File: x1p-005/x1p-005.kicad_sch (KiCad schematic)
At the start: 72 parts, among them Q1 LMBT3904LT1G, SW1 6.0*6.0*6.0, SW2 6.0*6.0*6.0, U1 AD24C02, U2 SN74LVC1T45DBVR, U4 SN74LVC1G3157DBVR_C3040658, U5 SN74LVC1G3157DBVR_C3040658

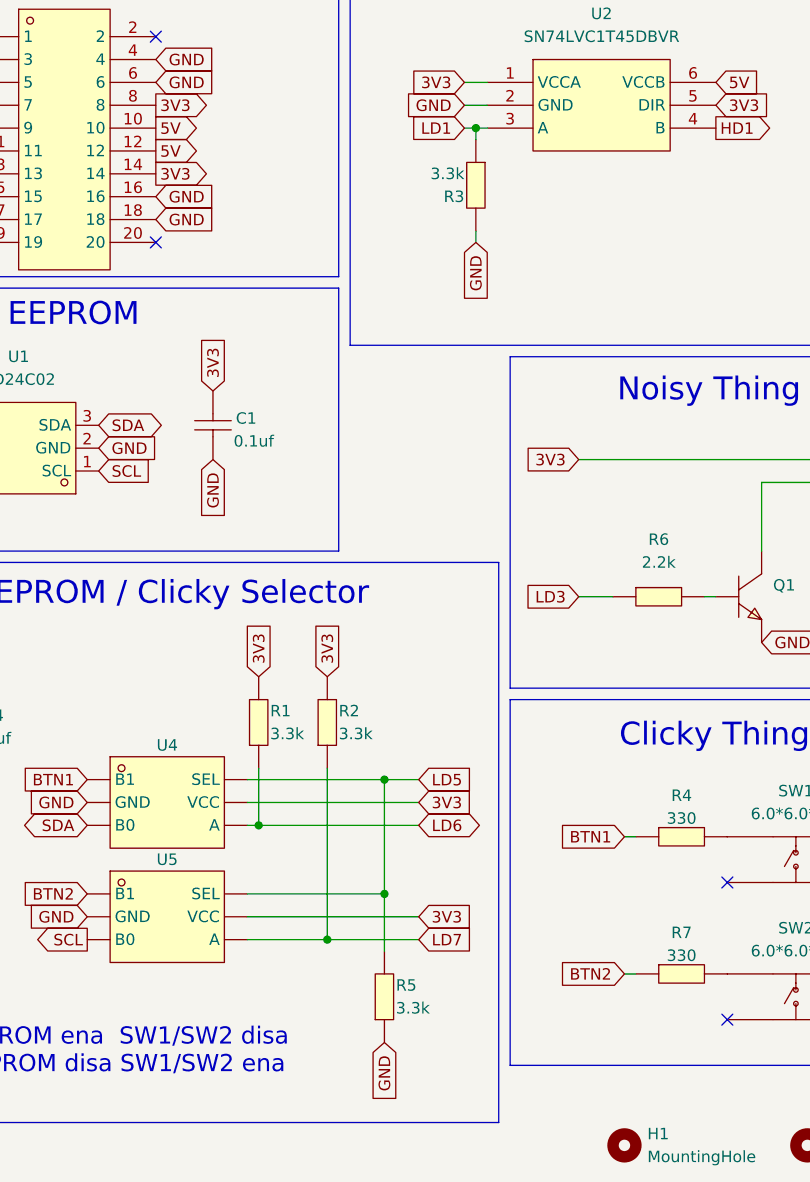
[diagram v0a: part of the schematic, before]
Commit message: x1p-005: resistors to 2.2k; remove a weird dangling trace; label beepies and clickies with their pin number
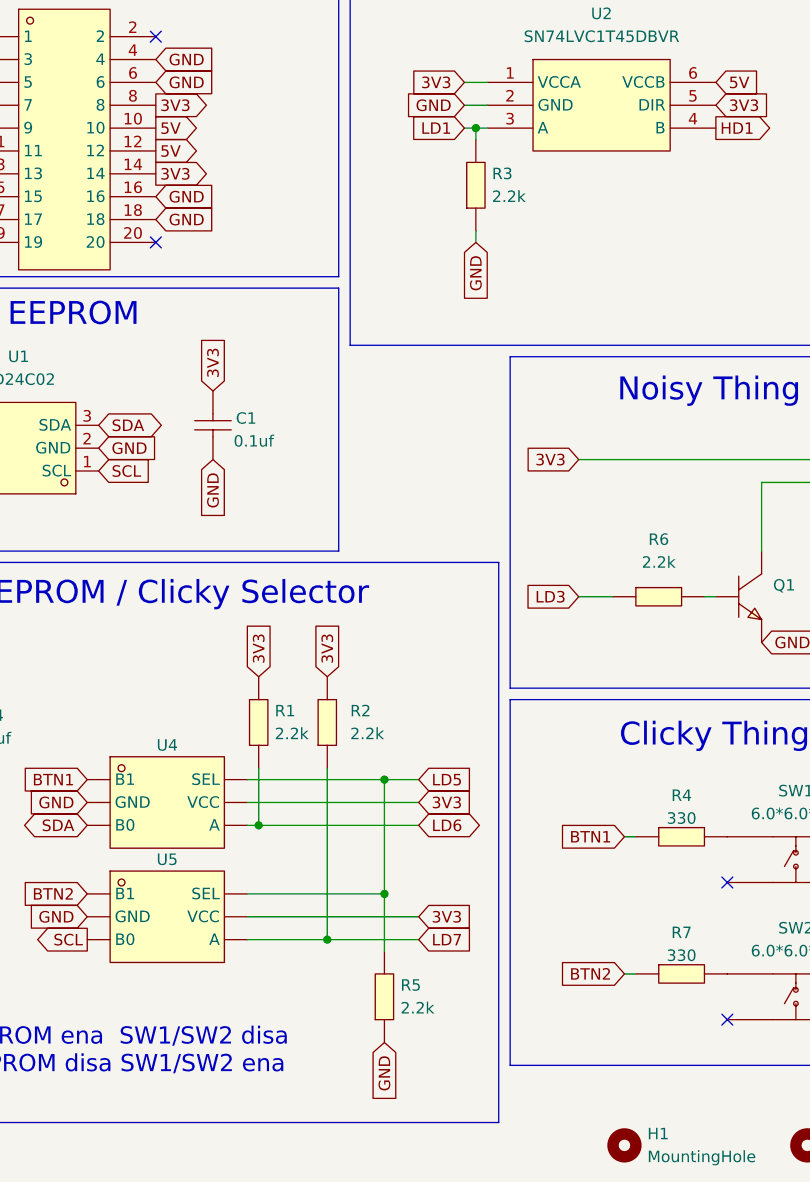
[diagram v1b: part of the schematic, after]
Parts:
- removed R1, R2, R5: 3.3k, x1p-005:R0402, symbol lcsc:0402WGF3301TCE
- removed R3: 3.3k, x1p-004:R0402, symbol lcsc:0402WGF3301TCE
- added R1, R2, R3, R5: 2.2k, x1p-005:R0402, symbol x1p-005:0402WGF2201TCE
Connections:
- net 3V3: now also R1.2, R2.2
- net GND: now also R3.1, R5.1
- net LD1: now also R3.2
- net LD5: now also R5.2
- net LD6: now also R1.1
- net LD7: now also R2.1

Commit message: x1p-005: fix up board layout to align with x1p-004
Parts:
- C1, C13, C14: footprint x1p-005:C0402 -> Capacitor_SMD:C_0402_1005Metric
- C10, C11, C12, C15, C16, C17, C18, C19, C2, C20, C21, C22, C23, C24, C25, C26, C27, C28, C29, C3, C4, C5, C6, C7, C8, C9: footprint x1p-004:C0402 -> Capacitor_SMD:C_0402_1005Metric
- R1, R2, R3, R4, R5, R6, R7: footprint x1p-005:R0402 -> Resistor_SMD:R_0402_1005Metric
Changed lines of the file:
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@@
 			)
 		)
-		(property "Footprint" "x1p-004:C0402"
+		(property "Footprint" "Capacitor_SMD:C_0402_1005Metric"
 			(at 204.47 137.16 0)
 			(effects
@@
 			)
 		)
-		(property "Footprint" "x1p-005:C0402"
+		(property "Footprint" "Capacitor_SMD:C_0402_1005Metric"
 			(at 19.05 101.6 0)
 			(effects
@@
 			)
 		)
-		(property "Footprint" "x1p-004:C0402"
+		(property "Footprint" "Capacitor_SMD:C_0402_1005Metric"
 			(at 247.65 137.16 0)
 			(effects
@@
 			)
 		)
-		(property "Footprint" "x1p-004:C0402"
+		(property "Footprint" "Capacitor_SMD:C_0402_1005Metric"
 			(at 166.37 137.16 0)
 			(effects
@@
 			)
 		)
-		(property "Footprint" "x1p-004:C0402"
+		(property "Footprint" "Capacitor_SMD:C_0402_1005Metric"
 			(at 166.37 149.86 0)
 			(effects
@@
 			)
 		)
-		(property "Footprint" "x1p-005:R0402"
+		(property "Footprint" "Resistor_SMD:R_0402_1005Metric"
 			(at 82.55 132.08 0)
 			(effects
@@
 			)
 		)
-		(property "Footprint" "x1p-004:C0402"
+		(property "Footprint" "Capacitor_SMD:C_0402_1005Metric"
 			(at 220.98 137.16 0)
 			(effects
@@
 			)
 		)
-		(property "Footprint" "x1p-004:C0402"
+		(property "Footprint" "Capacitor_SMD:C_0402_1005Metric"
 			(at 121.92 26.67 0)
 			(effects
@@
 			)
 		)
-		(property "Footprint" "x1p-004:C0402"
+		(property "Footprint" "Capacitor_SMD:C_0402_1005Metric"
 			(at 247.65 149.86 0)
 			(effects
@@
 			)
 		)
-		(property "Footprint" "x1p-005:R0402"
+		(property "Footprint" "Resistor_SMD:R_0402_1005Metric"
 			(at 92.71 41.91 0)
 			(effects
@@
 			)
 		)
-		(property "Footprint" "x1p-004:C0402"
+		(property "Footprint" "Capacitor_SMD:C_0402_1005Metric"
 			(at 189.23 137.16 0)
 			(effects
@@
 			)
 		)
-		(property "Footprint" "x1p-004:C0402"
+		(property "Footprint" "Capacitor_SMD:C_0402_1005Metric"
 			(at 256.54 149.86 0)
 			(effects
@@
 			)
 		)
-		(property "Footprint" "x1p-005:R0402"
+		(property "Footprint" "Resistor_SMD:R_0402_1005Metric"
 			(at 76.2 101.6 0)
 			(effects
@@
 			)
 		)
-		(property "Footprint" "x1p-004:C0402"
+		(property "Footprint" "Capacitor_SMD:C_0402_1005Metric"
 			(at 181.61 137.16 0)
 			(effects
@@
 			)
 		)
-		(property "Footprint" "x1p-005:R0402"
+		(property "Footprint" "Resistor_SMD:R_0402_1005Metric"
 			(at 107.95 137.16 0)
 			(effects
@@
 			)
 		)
-		(property "Footprint" "x1p-004:C0402"
+		(property "Footprint" "Capacitor_SMD:C_0402_1005Metric"
 			(at 220.98 149.86 0)
 			(effects
@@
 			)
 		)
-		(property "Footprint" "x1p-005:C0402"
+		(property "Footprint" "Capacitor_SMD:C_0402_1005Metric"
 			(at 10.16 101.6 0)
 			(effects
@@
 			)
 		)
-		(property "Footprint" "x1p-004:C0402"
+		(property "Footprint" "Capacitor_SMD:C_0402_1005Metric"
 			(at 158.75 149.86 0)
 			(effects
@@
 			)
 		)
-		(property "Footprint" "x1p-004:C0402"
+		(property "Footprint" "Capacitor_SMD:C_0402_1005Metric"
 			(at 189.23 149.86 0)
 			(effects
@@
 			)
 		)
-		(property "Footprint" "x1p-005:C0402"
+		(property "Footprint" "Capacitor_SMD:C_0402_1005Metric"
 			(at 48.26 68.58 0)
 			(effects
@@
 			)
 		)
-		(property "Footprint" "x1p-004:C0402"
+		(property "Footprint" "Capacitor_SMD:C_0402_1005Metric"
 			(at 204.47 149.86 0)
 			(effects
@@
 			)
 		)
-		(property "Footprint" "x1p-004:C0402"
+		(property "Footprint" "Capacitor_SMD:C_0402_1005Metric"
 			(at 212.09 137.16 0)
 			(effects
@@
 			)
 		)
-		(property "Footprint" "x1p-004:C0402"
+		(property "Footprint" "Capacitor_SMD:C_0402_1005Metric"
 			(at 212.09 149.86 0)
 			(effects
@@
 			)
 		)
-		(property "Footprint" "x1p-004:C0402"
+		(property "Footprint" "Capacitor_SMD:C_0402_1005Metric"
 			(at 238.76 149.86 0)
 			(effects
@@
 			)
 		)
-		(property "Footprint" "x1p-005:R0402"
+		(property "Footprint" "Resistor_SMD:R_0402_1005Metric"
 			(at 105.41 95.25 0)
 			(effects
@@
 			)
 		)
-		(property "Footprint" "x1p-004:C0402"
+		(property "Footprint" "Capacitor_SMD:C_0402_1005Metric"
 			(at 196.85 149.86 0)
 			(effects
@@
 			)
 		)
-		(property "Footprint" "x1p-004:C0402"
+		(property "Footprint" "Capacitor_SMD:C_0402_1005Metric"
 			(at 181.61 149.86 0)
 			(effects
@@
 			)
 		)
-		(property "Footprint" "x1p-005:R0402"
+		(property "Footprint" "Resistor_SMD:R_0402_1005Metric"
 			(at 68.58 101.6 0)
 			(effects
@@
 			)
 		)
-		(property "Footprint" "x1p-004:C0402"
+		(property "Footprint" "Capacitor_SMD:C_0402_1005Metric"
 			(at 229.87 137.16 0)
 			(effects
@@
 			)
 		)
-		(property "Footprint" "x1p-005:R0402"
+		(property "Footprint" "Resistor_SMD:R_0402_1005Metric"
 			(at 107.95 121.92 0)
 			(effects
@@
 			)
 		)
-		(property "Footprint" "x1p-004:C0402"
+		(property "Footprint" "Capacitor_SMD:C_0402_1005Metric"
 			(at 196.85 137.16 0)
 			(effects
@@
 			)
 		)
-		(property "Footprint" "x1p-004:C0402"
+		(property "Footprint" "Capacitor_SMD:C_0402_1005Metric"
 			(at 238.76 137.16 0)
 			(effects
@@
 			)
 		)
-		(property "Footprint" "x1p-004:C0402"
+		(property "Footprint" "Capacitor_SMD:C_0402_1005Metric"
 			(at 173.99 149.86 0)
 			(effects
@@
 			)
 		)
-		(property "Footprint" "x1p-004:C0402"
+		(property "Footprint" "Capacitor_SMD:C_0402_1005Metric"
 			(at 158.75 137.16 0)
 			(effects
@@
 			)
 		)
-		(property "Footprint" "x1p-004:C0402"
+		(property "Footprint" "Capacitor_SMD:C_0402_1005Metric"
 			(at 173.99 137.16 0)
 			(effects
@@
 			)
 		)
-		(property "Footprint" "x1p-004:C0402"
+		(property "Footprint" "Capacitor_SMD:C_0402_1005Metric"
 			(at 229.87 149.86 0)
 			(effects
